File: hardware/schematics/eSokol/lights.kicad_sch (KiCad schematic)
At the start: 47 parts, among them Q1 AO3400A, Q15 AO3401A, Q16 AO3400A, Q17 AO3401A, Q2 AO3400A, Q3 AO3400A, Q6 AO3401A, Q7 AO3401A, Q9 AO3400A, SW3 BRAKE, SW4 SW_BLINKERS, SW5 EMERG_BULBS, U1 hw-045 20V step-up

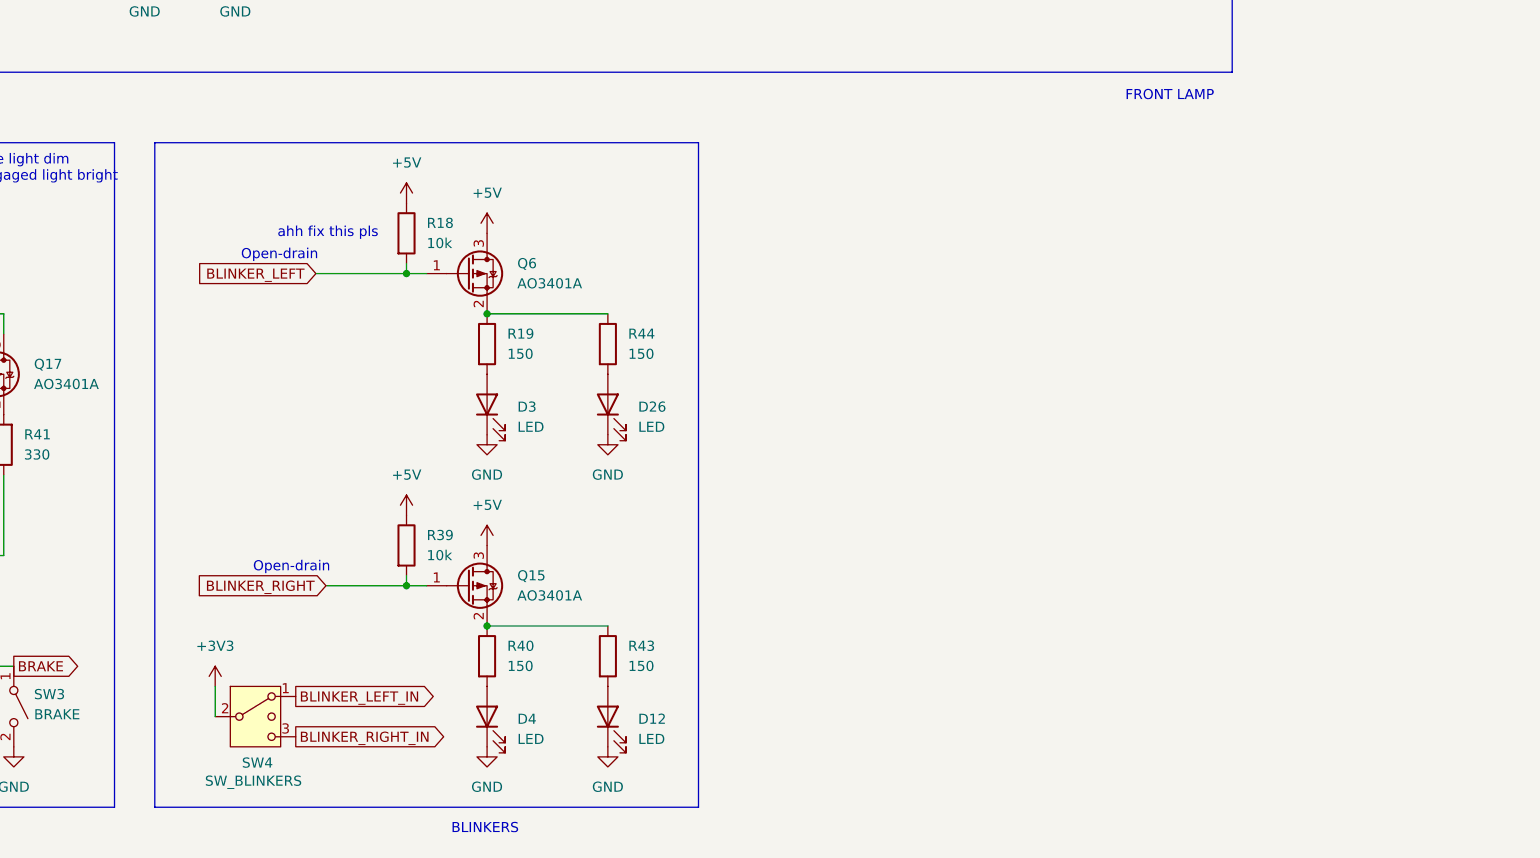
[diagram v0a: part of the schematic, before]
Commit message: WIP: update some schematics to reflect the newest design changes
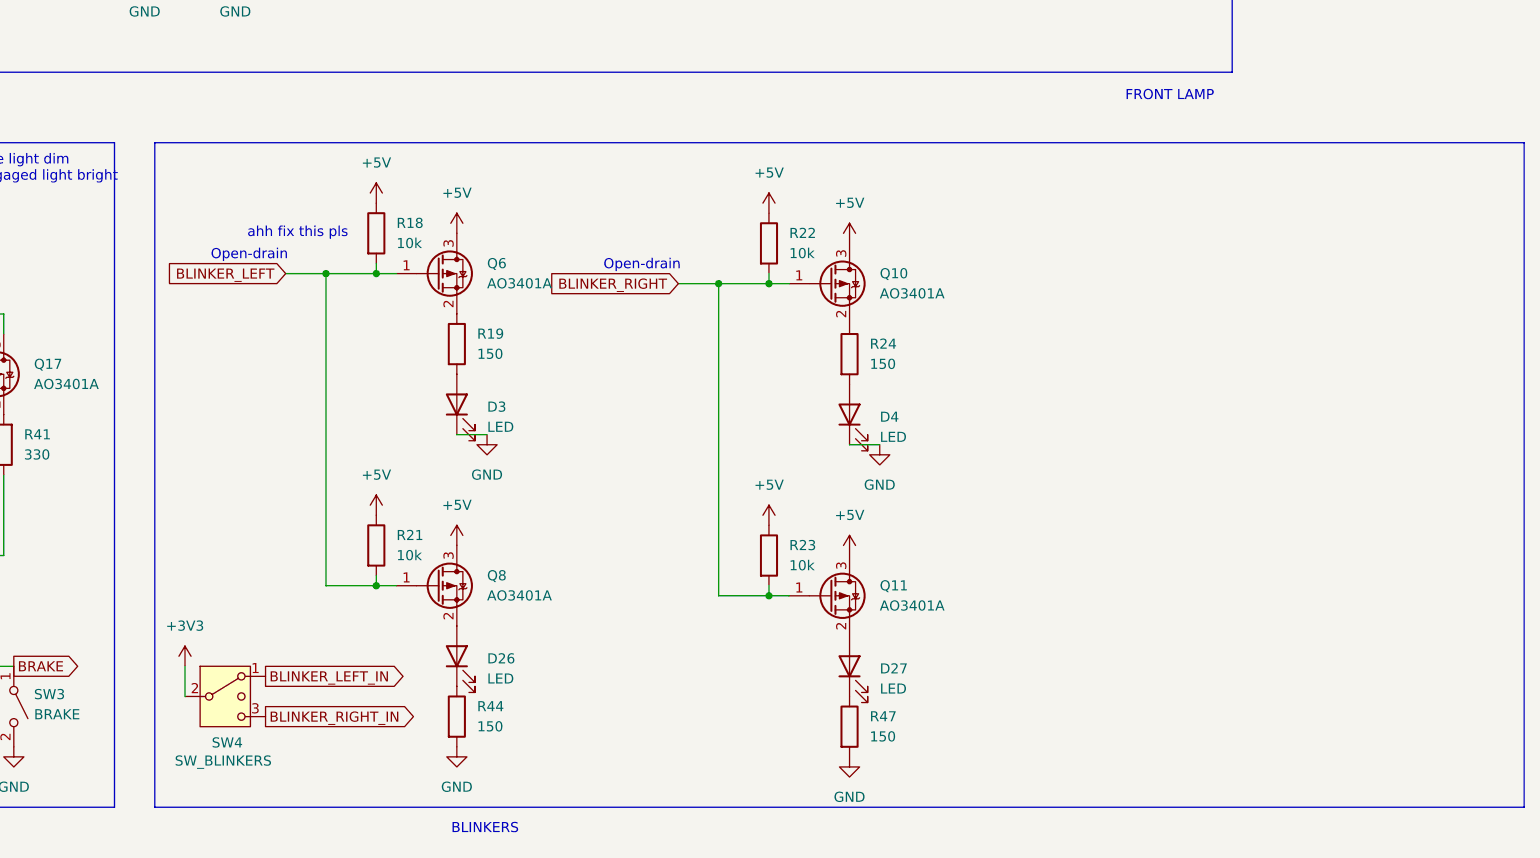
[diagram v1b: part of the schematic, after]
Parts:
- removed D12: LED, symbol Device:LED
- removed Q15: AO3401A, Package_TO_SOT_SMD:SOT-23, symbol Transistor_FET:AO3401A
- removed R39: 10k, symbol Device:R
- removed R40, R43: 150, symbol Device:R
- added D27: LED, symbol Device:LED
- added Q10, Q11, Q8: AO3401A, Package_TO_SOT_SMD:SOT-23, symbol Transistor_FET:AO3401A
- added R21, R22, R23: 10k, symbol Device:R
- added R24, R47: 150, symbol Device:R
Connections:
- net +5V: now also Q10.3 (D), Q11.3 (D), Q8.3 (D), R21.1, R22.1, R23.1
- net BLINKER_LEFT: now also Q8.1 (G), R21.2
- net BLINKER_RIGHT: now also Q10.1 (G), Q11.1 (G), R22.2, R23.2
- net GND: now also R44.2, R47.2; no longer D26.1 (K)
- net at Q6.2 (S), R19.1: no longer R44.1
- net at D4.2 (A): now also R24.2
- net at D26.2 (A): now also Q8.2 (S); no longer R44.2
- new net: Q10.2 (S), R24.1
- new net: D27.1 (K), R47.1
- new net: D27.2 (A), Q11.2 (S)
- new net: D26.1 (K), R44.1
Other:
- moved on the sheet: D26, D3, Q6, R18, R19, R44, SW4
